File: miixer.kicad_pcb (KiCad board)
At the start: 2 copper layers, 60 x 30 mm, 8 parts, among them J1 USB_C_Receptacle_USB2.0_16P, U1 ESP32-C3-WROOM-02, U3 USBLC6-2SC6

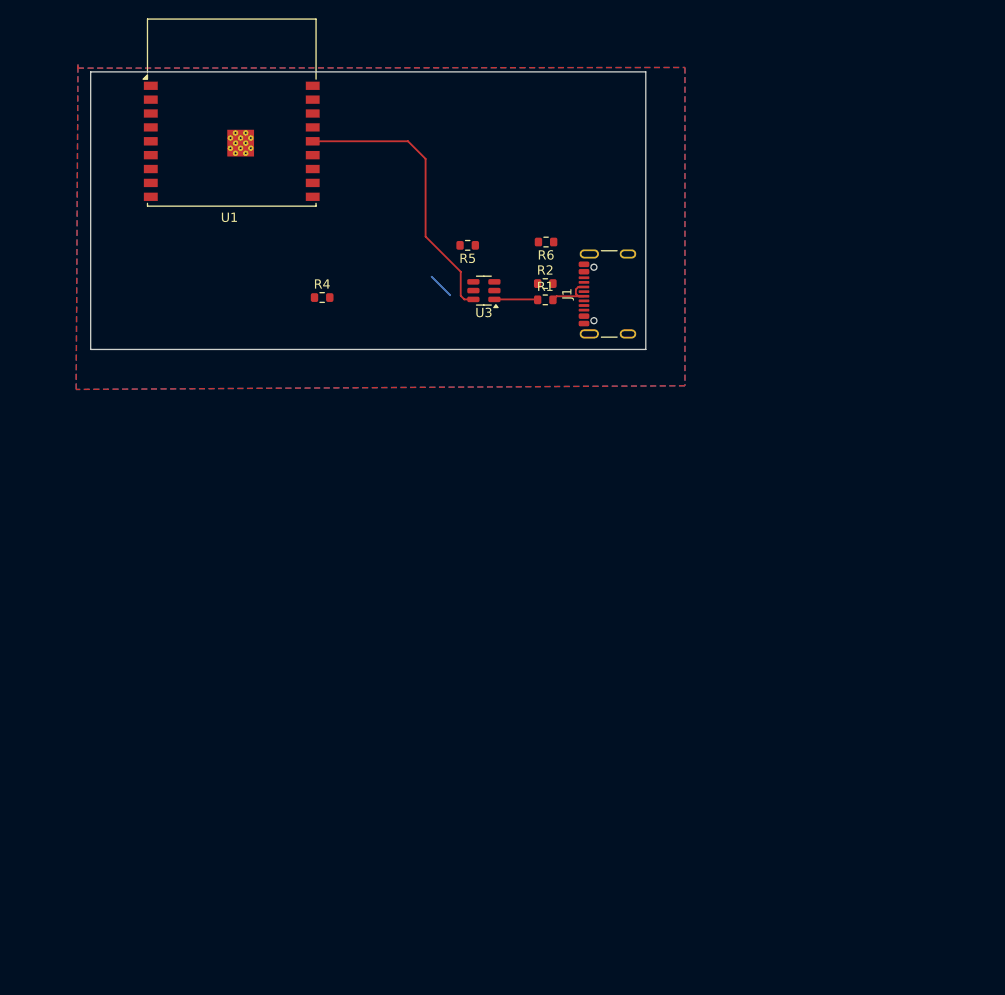
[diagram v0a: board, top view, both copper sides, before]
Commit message: Update
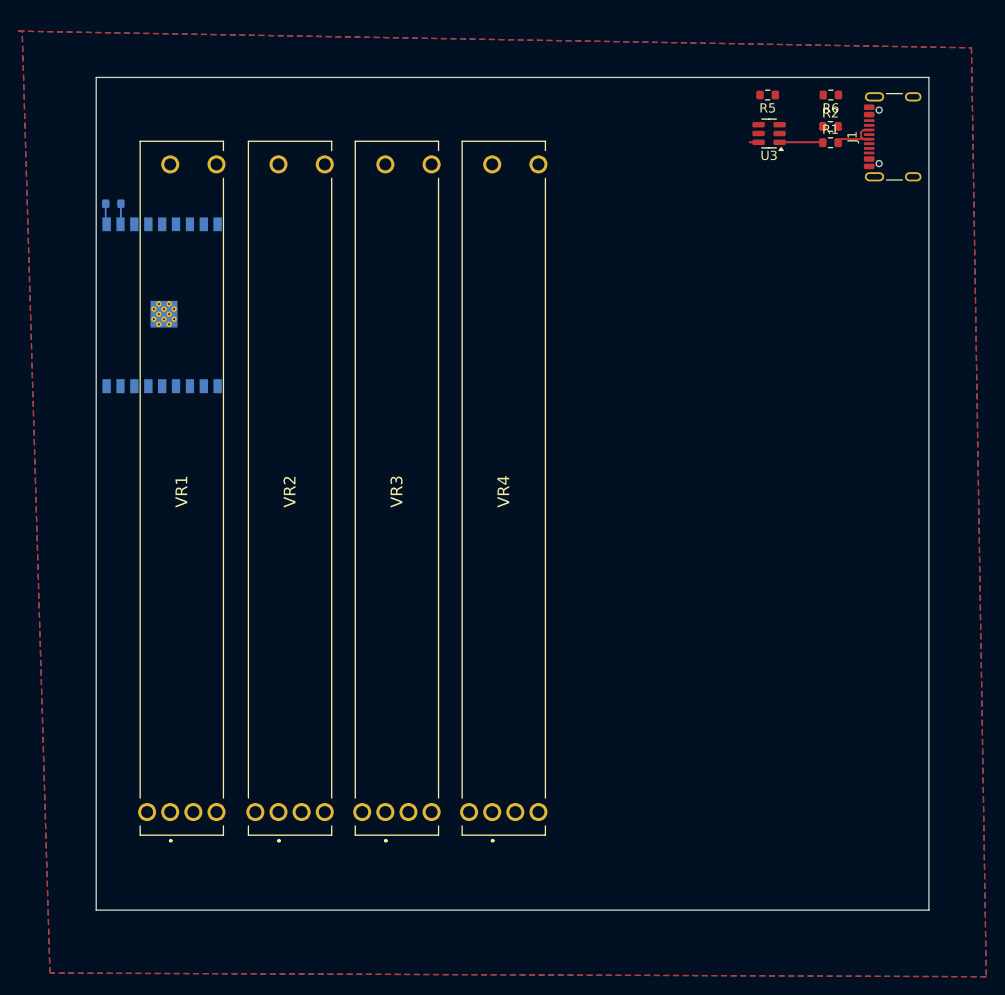
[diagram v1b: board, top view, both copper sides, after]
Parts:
- added VR1: PTL60-15G1-103B2, 00_Luc:PTL6015G1103B2, F.Cu at (38.6, 110.0)
- added VR2: PTL60-15G1-103B2, 00_Luc:PTL6015G1103B2, F.Cu at (50.3, 110.0)
- added VR3: PTL60-15G1-103B2, 00_Luc:PTL6015G1103B2, F.Cu at (61.9, 110.0)
- added VR4: PTL60-15G1-103B2, 00_Luc:PTL6015G1103B2, F.Cu at (73.4, 110.0)
- R4, U1: moved to B.Cu
- moved R5 36.3 mm to (103.2, 32.5)
- moved J1 35.2 mm to (117.8, 37.0)
- moved R1 35.2 mm to (110.0, 37.7)
- moved R2 35.2 mm to (110.0, 35.9)
- moved U3 35.2 mm to (103.3, 36.7)
- moved R6 34.6 mm to (110.0, 32.5)
- moved R4 24.7 mm to (32.5, 44.2), turned to 180 degrees
- moved U1 19.3 mm to (37.7, 55.2), turned to -90 degrees
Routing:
- net /MCU/USB_D+: track 30.9 -> 0.97 mm
- net VBUS: track 2.83 -> 0.00 mm
- net +3.3V: track 0.00 -> 2.27 mm
- net /MCU/ENABLE: track 0.00 -> 2.25 mm
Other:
- board size 60 x 30 mm -> 90 x 90 mm
